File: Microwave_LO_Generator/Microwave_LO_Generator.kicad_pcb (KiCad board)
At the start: 4 copper layers, 53.3 x 42.9 mm, 76 parts, among them J1 Conn_01x02_Male, J2 Conn_01x02_Male, J3 Conn_01x02_Female, J4 Conn_01x05_Male, J5 Conn_01x02_Female, U1 ADF4150HV, U2 LT1962-3.3, U3 LT3010, U4 HMC739LP4E, U5 LT1962-5, U6 LT1962-5, X1 IQXT-220-1

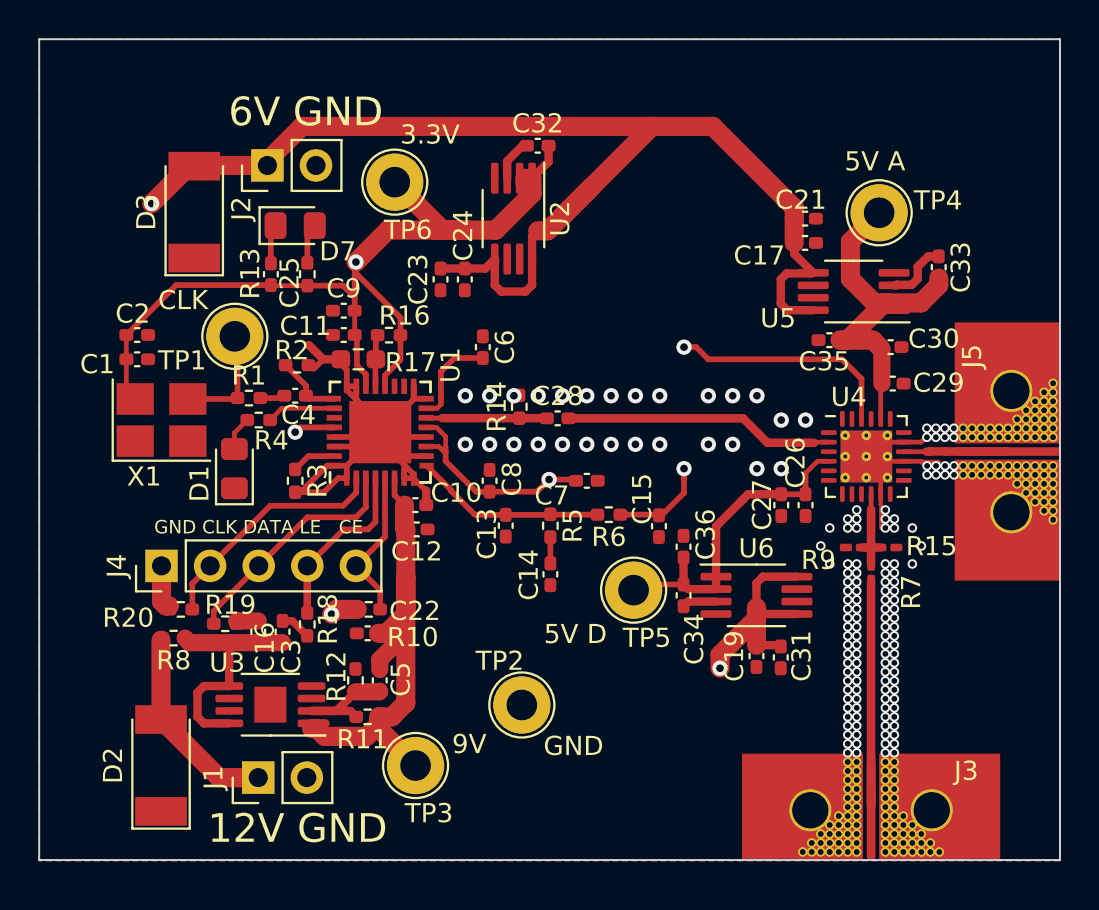
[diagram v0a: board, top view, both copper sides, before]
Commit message: Update
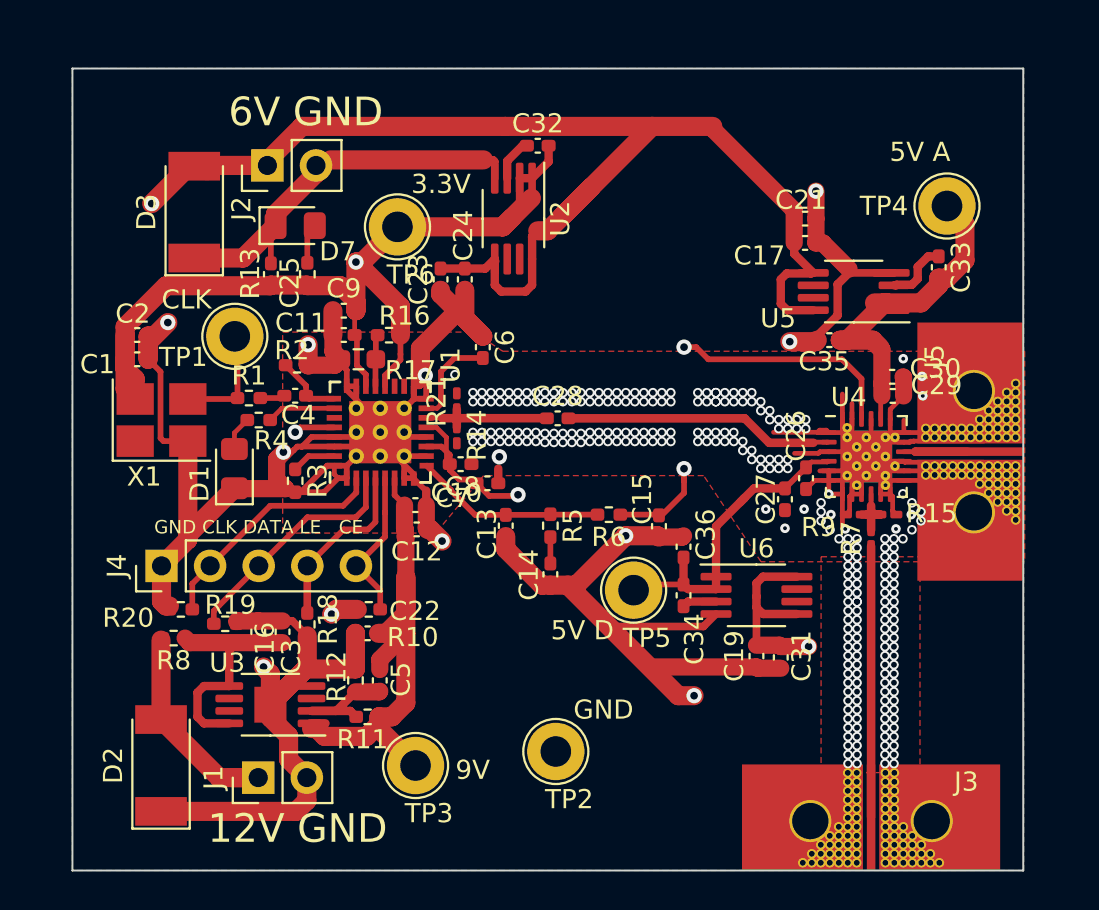
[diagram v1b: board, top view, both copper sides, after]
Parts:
- added R21: 100r, Microwave_LO_Generator:R_0201_0603_HandSolder_mod, F.Cu at (112.3, 97.3)
- R14: value 51r -> 100r; footprint Resistor_SMD:R_0402_1005Metric_Pad0.72x0.64mm_HandSolder -> Microwave_LO_Generator:R_0201_0603_HandSolder_mod
- moved C7 5.20 mm to (113.9, 101.6)
- moved R14 3.59 mm to (112.3, 99.1), turned to 270 degrees
- moved TP4 3.56 mm to (137.9, 87.1)
- moved TP2 3.01 mm to (117.5, 115.6)
- moved TP6 2.34 mm to (109.2, 88.2)
- moved J5 1.96 mm to (139.8, 99.9)
- moved R7 1.81 mm to (134.0, 104.5)
- moved C8 1.75 mm to (112.5, 100.6), turned to 180 degrees
- moved R15 1.72 mm to (134.9, 103.2)
- moved R9 1.72 mm to (133.1, 103.2)
- moved C30 1.55 mm to (135.1, 96.0)
- moved C26 1.41 mm to (130.6, 101.3)
- moved C29 0.64 mm to (135.1, 97.0)
- moved J3 0.56 mm to (134.1, 119.7)
- moved C27 0.36 mm to (129.5, 102.5)
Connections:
- U4 pad 1: (no net) -> 0
- U4 pad 12: (no net) -> 0
- U4 pad 13: (no net) -> 0
- U4 pad 14: (no net) -> 0
- U4 pad 18: (no net) -> 0
- U4 pad 19: (no net) -> 0
- U4 pad 21: (no net) -> 0
- U4 pad 23: (no net) -> 0
- U4 pad 24: (no net) -> 0
- U4 pad 3: (no net) -> 0
- U4 pad 5: (no net) -> 0
- U4 pad 6: (no net) -> 0
- U4 pad 7: (no net) -> 0
- U4 pad 8: (no net) -> 0
- U4 pad 9: (no net) -> 0
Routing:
- net 0: track 61.3 -> 280.8 mm, vias 147 -> 281
- net +3V3: track 109.1 -> 134.6 mm
- net DIV16: track 6.55 -> 8.17 mm
- net Net-(J5-Pad1): track 5.42 -> 4.13 mm
- net Net-(J3-Pad1): track 14.9 -> 14.2 mm
- net Net-(R15-Pad1): track 4.68 -> 3.96 mm
- net +5VD: track 17.5 -> 16.9 mm
- net +6V: track 137.0 -> 136.5 mm
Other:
- board size 53.3 x 42.9 mm -> 49.7 x 41.9 mm
